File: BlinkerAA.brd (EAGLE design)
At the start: 55.9 x 15.2 mm, 19 parts, among them IC1 LMV611MGX_NOPB

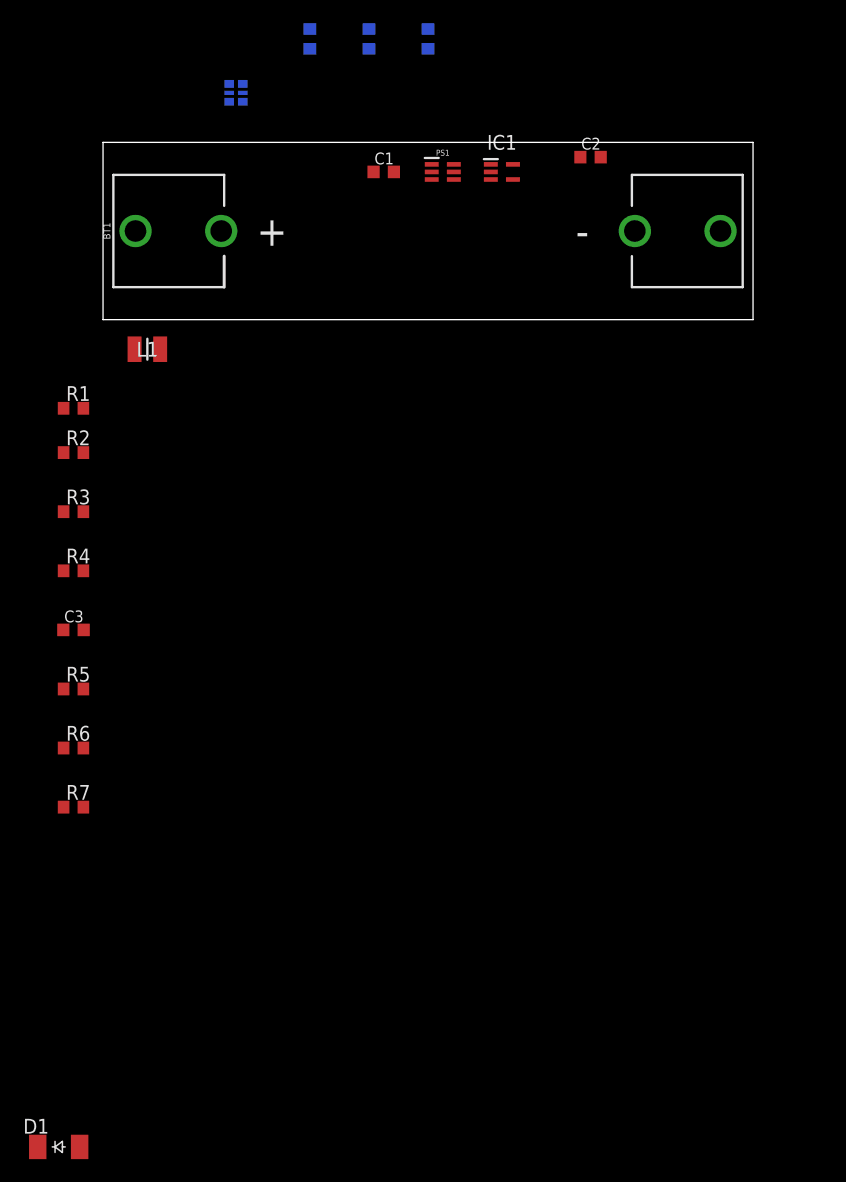
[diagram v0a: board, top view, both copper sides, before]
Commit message: gerbers generation, readme update
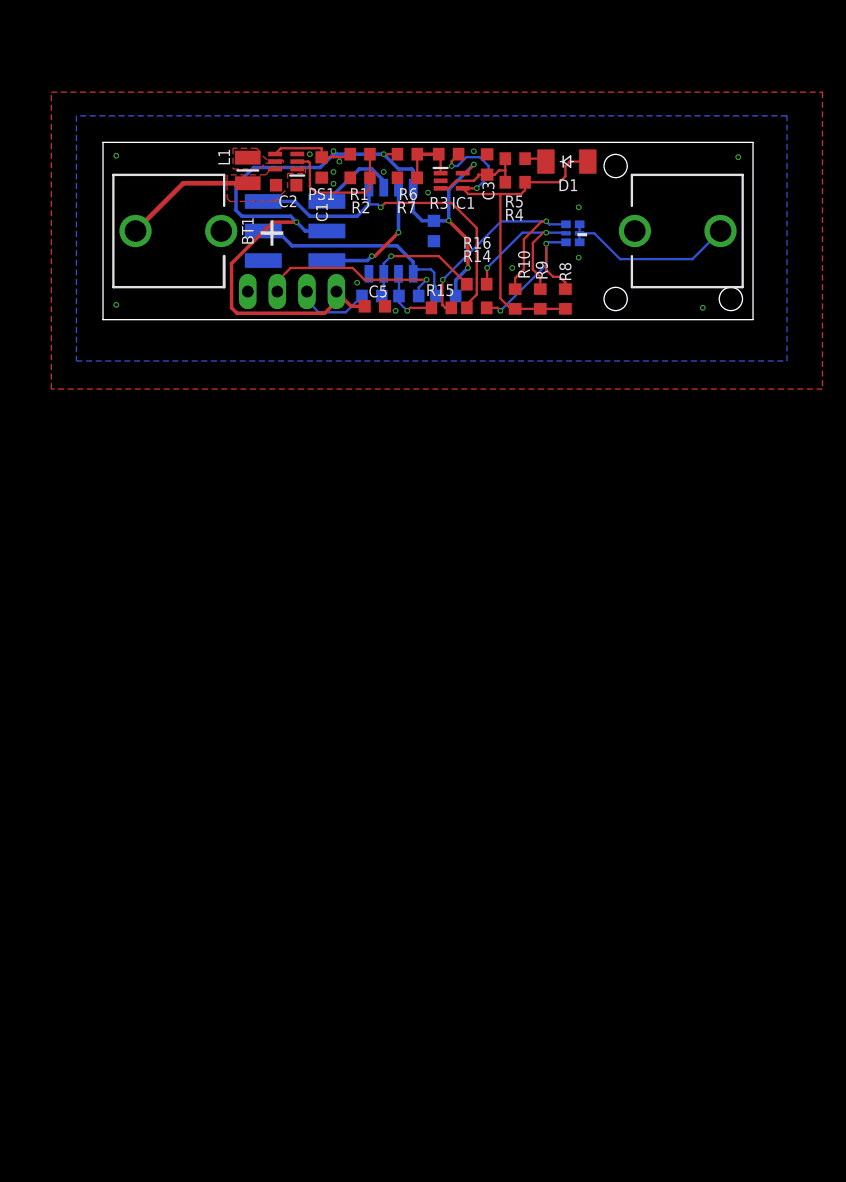
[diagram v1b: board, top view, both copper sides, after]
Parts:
- added C4, C5: 10u, resistor:C0603K
- added J1: 10129383-906001ALF, SamacSys_Parts:10129383906001ALF
- added JP1: (no value), pinhead:1X04
- added R11: 2.2M, rcl:R0603
- added R12, R13: 0, rcl:R0603
- added R14, R15, R16: DNI, rcl:R0603
- added U1: ATTINY85, SparkFun-IC-Microcontroller:ATTINY85
- moved D1 95.3 mm to (39.9, 13.6)
- moved R7 61.2 mm to (26.2, 12.2), turned to 180 degrees
- moved R5 59.3 mm to (35.4, 13.8), turned to 180 degrees
- moved R6 58.6 mm to (26.2, 14.2)
- moved C3 53.5 mm to (33.0, 13.3), turned to 90 degrees
- moved R4 50.6 mm to (35.4, 11.8), turned to 180 degrees
- moved R3 44.6 mm to (29.7, 14.2), turned to 180 degrees
- moved R2 34.1 mm to (22.1, 12.2)
- moved R1 32.9 mm to (22.1, 14.2), turned to 180 degrees
- moved R8 31.3 mm to (39.8, 1.78), flipped to the top
- moved LED1 31.0 mm to (40.4, 7.87), turned to 90 degrees
- moved R9 26.8 mm to (37.6, 1.78), flipped to the top
- moved C2 26.3 mm to (15.7, 11.6)
- moved R10 23.6 mm to (35.4, 1.78), flipped to the top
- moved L1 17.6 mm to (12.4, 12.8), turned to 90 degrees
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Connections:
- net N$1 renamed VIN
- net N$5 renamed FB
- removed net N$6: LED1.1, R10.2
- removed net N$8: LED1.2, R9.2
- removed net N$9: LED1.3, R8.2
- new net LB: LED1.6, R10.1, R15.1
- new net LG: LED1.5, R16.1, R9.1
- new net LR: LED1.4, R14.1, R8.1
- new net MISO: J1.A1, U1.6
- new net MOSI: J1.B1, R14.2, U1.5
- new net PB3: R13.2, R15.2, U1.2
- new net PB3C: JP1.3, R13.1
- new net PB4: R12.2, R16.2, U1.3
- new net PB4C: JP1.2, R12.1
- new net RSTN: J1.B2, R11.1, U1.1
- new net SCK: J1.A3, U1.7
- net +3V3: now also C4.1, C5.1, J1.A2, JP1.1, R11.2, U1.8
- net GND: now also C4.2, C5.2, J1.B3, JP1.4, LED1.1, LED1.2, LED1.3, U1.4; no longer R10.1, R8.1, R9.1
- net N$4: now also R10.2, R8.2, R9.2; no longer LED1.4, LED1.5, LED1.6
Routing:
- net +3V3: track 0.00 -> 83.4 mm, vias 0 -> 7
- net N$4: track 0.00 -> 36.6 mm, vias 0 -> 2
- net MOSI: track 0.00 -> 29.1 mm, vias 0 -> 1
- net LB: track 0.00 -> 23.0 mm, vias 0 -> 2
- net RSTN: track 0.00 -> 19.2 mm
- net PB3C: track 0.00 -> 16.3 mm, vias 0 -> 1
- net GND: track 0.00 -> 15.6 mm, vias 0 -> 15
- net LR: track 0.00 -> 15.3 mm, vias 0 -> 2
- net LG: track 0.00 -> 15.2 mm, vias 0 -> 2
- net VIN: track 0.00 -> 11.9 mm
- net FB: track 0.00 -> 11.6 mm
- net PB4: track 0.00 -> 11.3 mm, vias 0 -> 1
- net SCK: track 0.00 -> 11.0 mm, vias 0 -> 2
- net N$7: track 0.00 -> 8.30 mm
- net MISO: track 0.00 -> 7.06 mm
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- added copper zone on layer 1, net GND
- added copper zone on layer 16, net GND
- added copper zone on layer 1, net N$3
- added copper zone on layer 1, net VIN
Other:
- board text added: "Electronics design solutions s.r.o."
- board text added: "Juraj Repčík"
